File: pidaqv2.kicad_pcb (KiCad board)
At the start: 2 copper layers, 66 x 66 mm, 20 parts, among them J1 Raspberry_Pi_2_3, U1 INA2126E_250, U2 ADS114S08BIPBS, U3 ADS114S08BIPBS

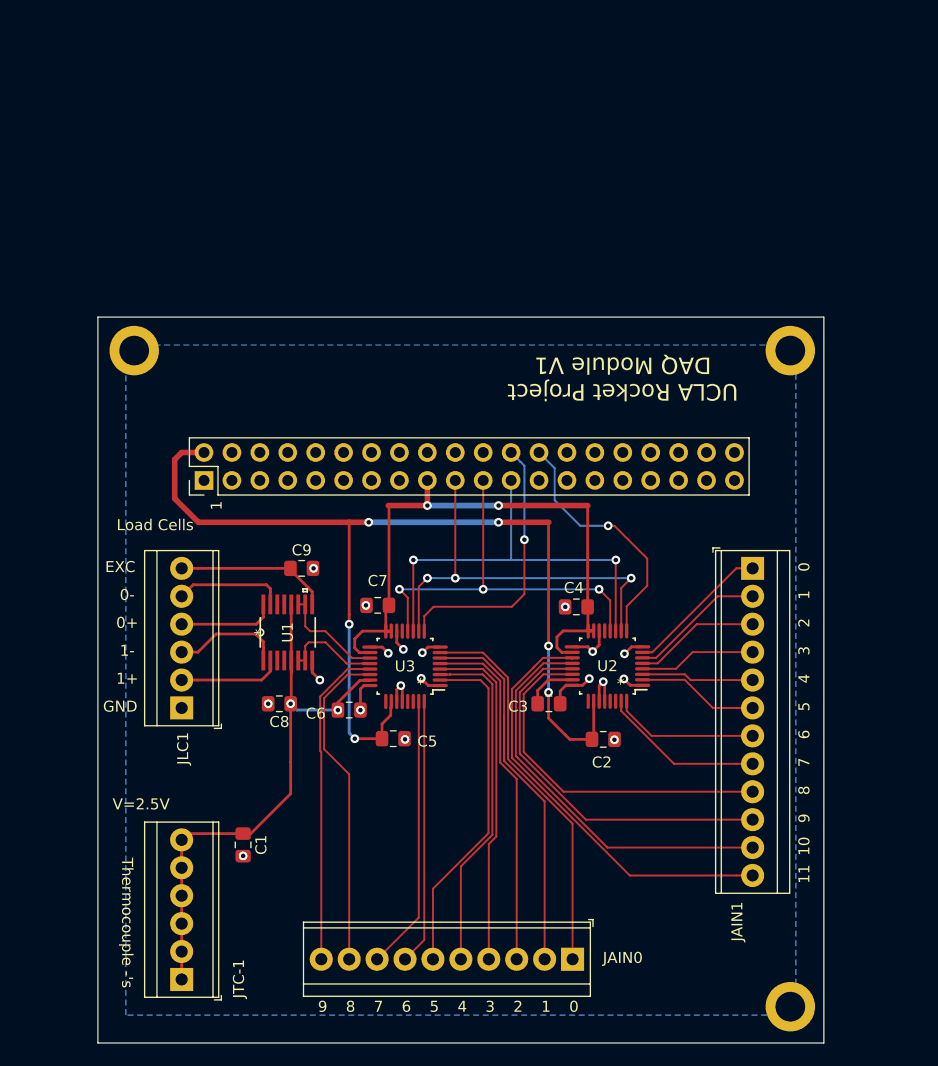
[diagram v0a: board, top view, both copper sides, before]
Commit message: ads1261
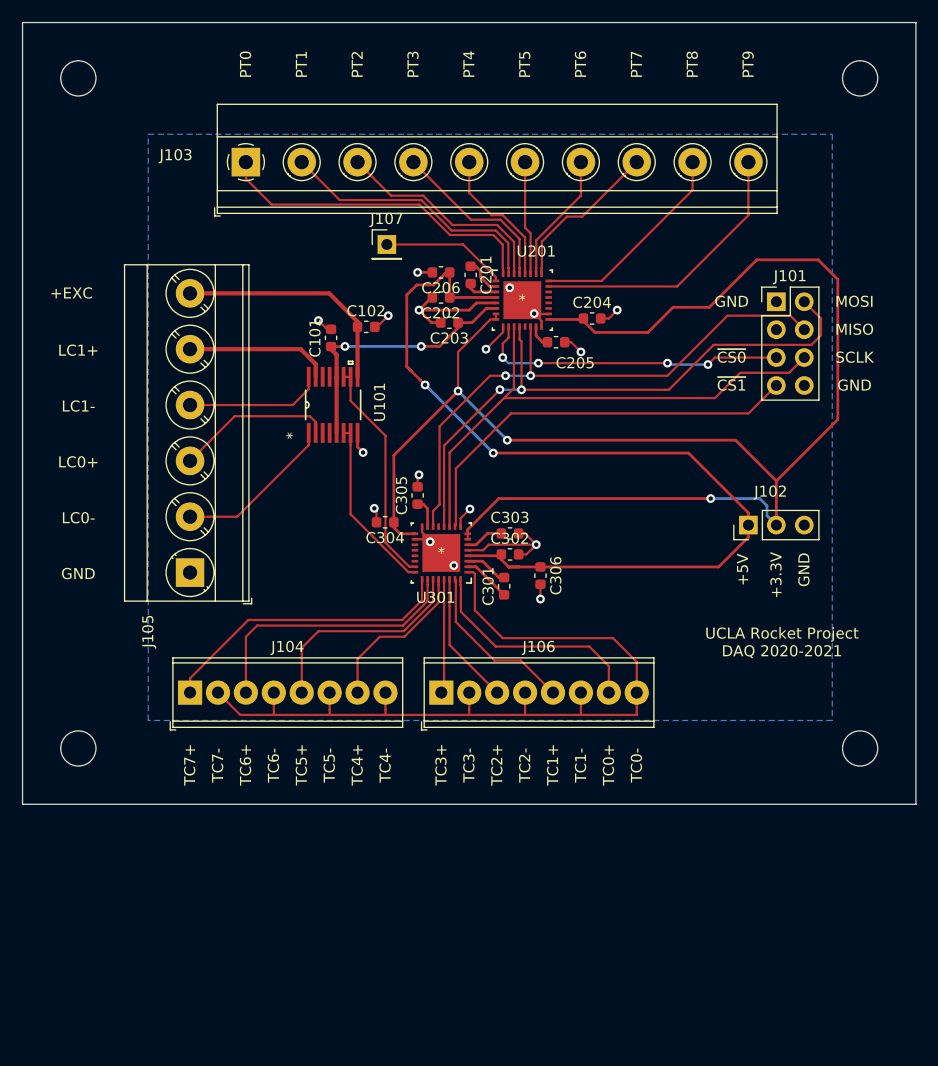
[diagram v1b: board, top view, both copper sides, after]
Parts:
- removed C1, C4, C7, C8, C9: 0.1uF, Capacitor_SMD:C_0805_2012Metric_Pad1.15x1.40mm_HandSolder
- removed C2, C5: 330nF, Capacitor_SMD:C_0805_2012Metric_Pad1.15x1.40mm_HandSolder
- removed C3, C6: 1uF, Capacitor_SMD:C_0805_2012Metric_Pad1.15x1.40mm_HandSolder
- removed J1: Raspberry_Pi_2_3, Connector_PinHeader_2.54mm:PinHeader_2x20_P2.54mm_Vertical
- removed JAIN0: Screw_Terminal_01x10, TerminalBlock_TE-Connectivity:TerminalBlock_TE_1-282834-0_1x10_P2.54mm_Horizontal
- removed JAIN1: Screw_Terminal_01x12, TerminalBlock_TE-Connectivity:TerminalBlock_TE_1-282834-2_1x12_P2.54mm_Horizontal
- removed JLC1, JTC-1: Screw_Terminal_01x06, TerminalBlock_TE-Connectivity:TerminalBlock_TE_282834-6_1x06_P2.54mm_Horizontal
- removed MK1, MK2, MK3: MountingHole_Pad, MountingHole:MountingHole_2.7mm_M2.5_ISO14580_Pad
- removed U1: INA2126E_250, footprints:INA2126E&slash_250
- removed U2, U3: ADS114S08BIPBS, footprints:ADS114S08BIPBS
- added C101: 0.1uF, Capacitor_SMD:C_0603_1608Metric, F.Cu at (124.6, 97.3)
- added C102: 0.1uF, Capacitor_SMD:C_0603_1608Metric, F.Cu at (127.8, 96.3)
- added C201: 4.7nF C0G, Capacitor_SMD:C_0603_1608Metric, F.Cu at (137.3, 91.5)
- added C202: 1uF, Capacitor_SMD:C_0603_1608Metric, F.Cu at (134.6, 93.6)
- added C203: 10uF, Capacitor_SMD:C_0603_1608Metric, F.Cu at (135.4, 95.9)
- added C204: 1uF, Capacitor_SMD:C_0603_1608Metric, F.Cu at (148.3, 95.5)
- added C205: 1uF, Capacitor_SMD:C_0603_1608Metric, F.Cu at (145.1, 97.7)
- added C206: 10uF, Capacitor_SMD:C_0603_1608Metric, F.Cu at (134.6, 91.3)
- added C301: 4.7nF C0G, Capacitor_SMD:C_0603_1608Metric, F.Cu at (140.3, 119.9)
- added C302: 1uF, Capacitor_SMD:C_0603_1608Metric, F.Cu at (140.9, 117.0)
- added C303: 10uF, Capacitor_SMD:C_0603_1608Metric, F.Cu at (140.9, 115.1)
- added C304: 1uF, Capacitor_SMD:C_0603_1608Metric, F.Cu at (129.5, 114.0)
- added C305: 1uF, Capacitor_SMD:C_0603_1608Metric, F.Cu at (132.5, 111.6)
- added C306: 10uF, Capacitor_SMD:C_0603_1608Metric, F.Cu at (143.6, 118.9)
- added H101: MountingHole, MountingHole:MountingHole_3.2mm_M3_ISO7380, F.Cu at (172.7, 134.6)
- added H102: MountingHole, MountingHole:MountingHole_3.2mm_M3_ISO7380, F.Cu at (101.6, 134.6)
- added H103: MountingHole, MountingHole:MountingHole_3.2mm_M3_ISO7380, F.Cu at (172.7, 73.7)
- added H104: MountingHole, MountingHole:MountingHole_3.2mm_M3_ISO7380, F.Cu at (101.6, 73.7)
- added J101: Conn_02x04_Odd_Even, Connector_PinHeader_2.54mm:PinHeader_2x04_P2.54mm_Vertical, F.Cu at (165.1, 94.0)
- added J102: Conn_01x03, Connector_PinHeader_2.54mm:PinHeader_1x03_P2.54mm_Vertical, F.Cu at (162.6, 114.3)
- added J103: Screw_Terminal_01x10, TerminalBlock_Phoenix:TerminalBlock_Phoenix_MKDS-1,5-10-5.08_1x10_P5.08mm_Horizontal, F.Cu at (116.8, 81.3)
- added J104: Screw_Terminal_01x08, TerminalBlock_Phoenix:TerminalBlock_Phoenix_MPT-0,5-8-2.54_1x08_P2.54mm_Horizontal, F.Cu at (111.8, 129.5)
- added J105: Screw_Terminal_01x06, TerminalBlock_Phoenix:TerminalBlock_Phoenix_MKDS-3-6-5.08_1x06_P5.08mm_Horizontal, F.Cu at (111.8, 118.6)
- added J106: Screw_Terminal_01x08, TerminalBlock_Phoenix:TerminalBlock_Phoenix_MPT-0,5-8-2.54_1x08_P2.54mm_Horizontal, F.Cu at (134.6, 129.5)
- added J107: Conn_01x01_Female, Connector_PinHeader_2.54mm:PinHeader_1x01_P2.54mm_Vertical, F.Cu at (129.7, 88.8)
- added U101: INA2126E_250, footprints:INA2126E&slash_250, F.Cu at (124.8, 103.4)
- added U201: ADS1261BIRHBR, footprints:ADS1261BIRHBR, F.Cu at (142.0, 93.8)
- added U301: ADS1261BIRHBR, footprints:ADS1261BIRHBR, F.Cu at (134.6, 116.8)
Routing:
- net +3V3: track 56.3 -> 145.3 mm, vias 2 -> 3
- net TC-: track 0.00 -> 76.7 mm
- net +2.5V: track 51.8 -> 0.00 mm, vias 2 -> 0
- net /ADC_Module/A11: track 39.3 -> 0.00 mm
- net /sheet5F3BC562/A1: track 38.4 -> 0.00 mm
- net ~CS1: track 0.00 -> 37.6 mm
- net /ADC_Module/A10: track 37.1 -> 0.00 mm
- net /sheet5F3BC562/A0: track 35.6 -> 0.00 mm
- net /ADC_Module/A9: track 34.9 -> 0.00 mm
- net /ADC_Module/A8: track 32.8 -> 0.00 mm
- net /sheet5F3BC562/A2: track 32.1 -> 0.00 mm
- net /sheet5F3BC562/A5: track 31.5 -> 0.00 mm
- net /sheet5F3BC562/A4: track 31.3 -> 0.00 mm
- net /sheet5F3BC562/A3: track 31.1 -> 0.00 mm
- net /ADC0/AIN0: track 0.00 -> 30.0 mm
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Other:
- board size 66 x 66 mm -> 81.3 x 71.1 mm
- net class Default: clearance 0.1778 -> 0.2032; trace_width 0.1778 -> 0.2032
- rule pad_to_mask_clearance: 0.051 -> 0
- rule trace_clearance: 0.1778 -> 0.2032
- rule trace_min: 0.1778 -> 0.2032
- rule via_min_drill: 0.3 -> 0.381
- rule via_min_size: 0.3048 -> 0.3302
- board text added: "+3.3V"
- board text added: "+5V"
- board text added: "+EXC"
- board text added: "LC0+"
- board text added: "LC0-"
- board text added: "LC1+"
- board text added: "LC1-"
- board text added: "MISO"
- board text added: "MOSI"
- board text added: "PT0"
- board text added: "PT1"
- board text added: "PT2"
- board text added: "PT3"
- board text added: "PT4"
- board text added: "PT5"
- board text added: "PT6"
- board text added: "PT7"
- board text added: "PT8"
- board text added: "PT9"
- board text added: "Raspi mounted here"
- board text added: "SCLK"
- board text added: "TC0+"
- board text added: "TC0-"
- board text added: "TC1+"
- board text added: "TC1-"
- board text added: "TC2+"
- board text added: "TC2-"
- board text added: "TC3+"
- board text added: "TC3-"
- board text added: "TC4+"
- board text added: "TC4-"
- board text added: "TC5+"
- board text added: "TC5-"
- board text added: "TC6+"
- board text added: "TC6-"
- board text added: "TC7+"
- board text added: "TC7-"
- board text added: "UCLA Rocket Project DAQ 2020-2021"
- board text added: "~CS0"
- board text added: "~CS1"
- board text removed: "0"
- board text removed: "0+"
- board text removed: "0-"
- board text removed: "1"
- board text removed: "1+"
- board text removed: "1-"
- board text removed: "10"
- board text removed: "11"
- board text removed: "2"
- board text removed: "3"
- board text removed: "4"
- board text removed: "5"
- board text removed: "6"
- board text removed: "7"
- board text removed: "8"
- board text removed: "9"
- board text removed: "EXC"
- board text removed: "Load Cells"
- board text removed: "Thermocouple -'s"
- board text removed: "UCLA Rocket Project DAQ Module V1"
- board text removed: "V=2.5V"
